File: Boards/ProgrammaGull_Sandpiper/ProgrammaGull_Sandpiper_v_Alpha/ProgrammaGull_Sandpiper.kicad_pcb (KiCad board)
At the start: 4 copper layers, 100 x 75 mm, 191 parts, among them J4 Conn_01x22_Socket, P1 USB_C_Plug_USB2.0, Q1 MMBT2907, Q2 MMBT2907, Q3 MMBT2907, Q4 MMBT2907, Q5 MMBT2907, Q6 MMBT2907, Q7 MMBT2907, Q8 MMBT2907, SW10 SW_Push, SW11 SW_Push, SW12 SW_Push, SW14 SW_Push, SW9 SW_Push, U1 ICE40UP5K-SG48ITR, U11 ADC084S051CIMM/NOPB, U12 74HC596, U13 74AHC595, U14 W25Q32JVSS, U15 AMS1117-3.3, U2 SN74LVC1G126DCKR, U3 74HC596, U4 MIC5504-1.2YM5, U5 MIC5504-2.5YM5, U6 93LCxxAxxOT, U7 FT2232HQ, X1 SG-210STF

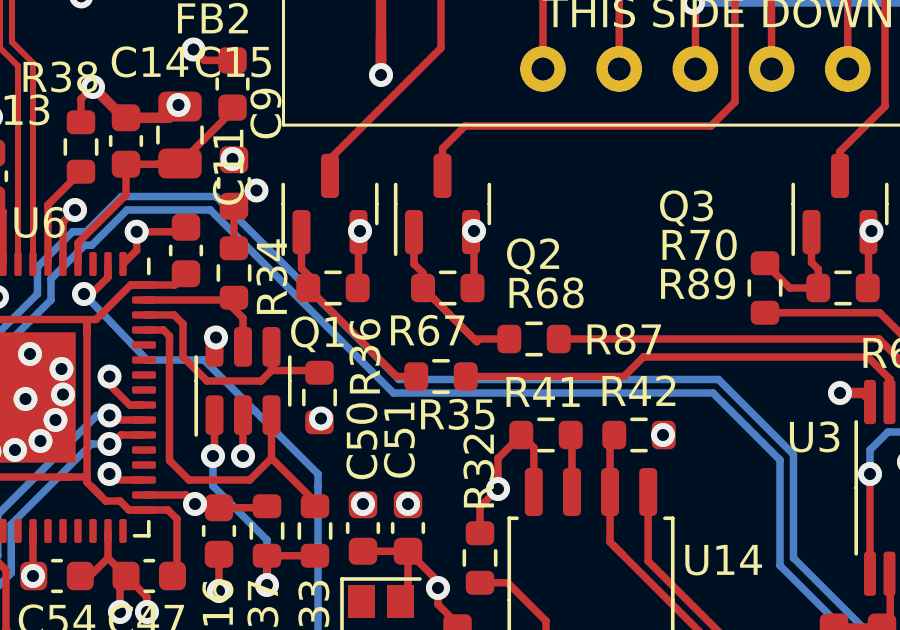
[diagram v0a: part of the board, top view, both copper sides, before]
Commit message: Minor Adds, small fixes on Sandpiper PCB
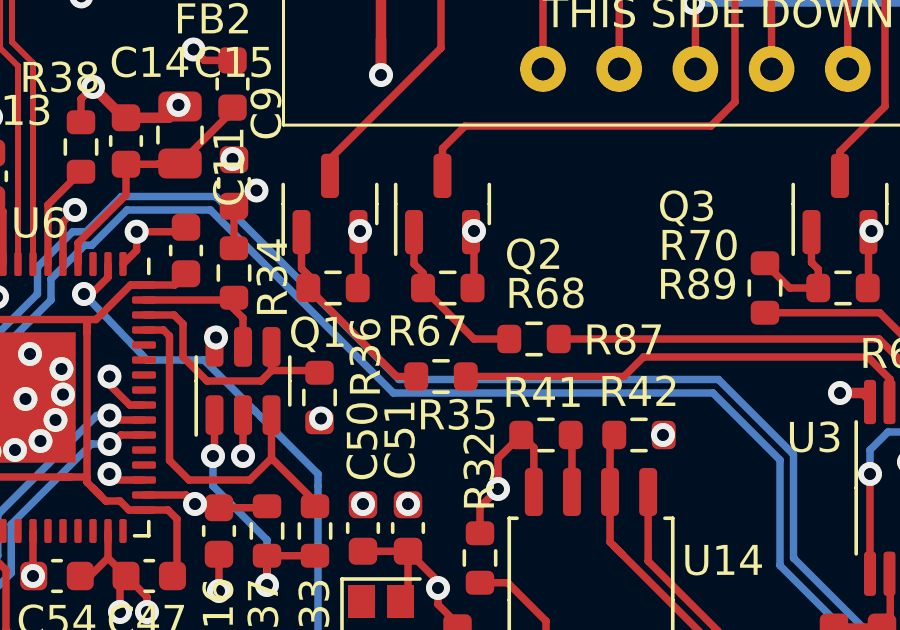
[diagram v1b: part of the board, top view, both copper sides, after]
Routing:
- net /UI_MSB_CA1: track 8.11 -> 5.57 mm
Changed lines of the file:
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@@
   (segment (start 50.2 31.5) (end 51.96 29.74) (width 0.25) (layer "F.Cu") (net 32))
   (segment (start 49.3 45.4375) (end 49.3 46.5) (width 0.25) (layer "F.Cu") (net 33))
-  (segment (start 51.4 49.1) (end 49.6 47.3) (width 0.25) (layer "F.Cu") (net 33))
   (segment (start 49.3 46.5) (end 49.6 46.8) (width 0.25) (layer "F.Cu") (net 33))
   (segment (start 49.6 46.8) (end 49.6 47.3) (width 0.25) (layer "F.Cu") (net 33))
